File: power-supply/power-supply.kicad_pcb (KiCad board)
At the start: 2 copper layers, 25 x 11.2 mm, 12 parts, among them J1 Conn_01x04, Q1 Q_PMOS_GSD, Q3 Q_NMOS_GSD, U1 AZ1084-5.0

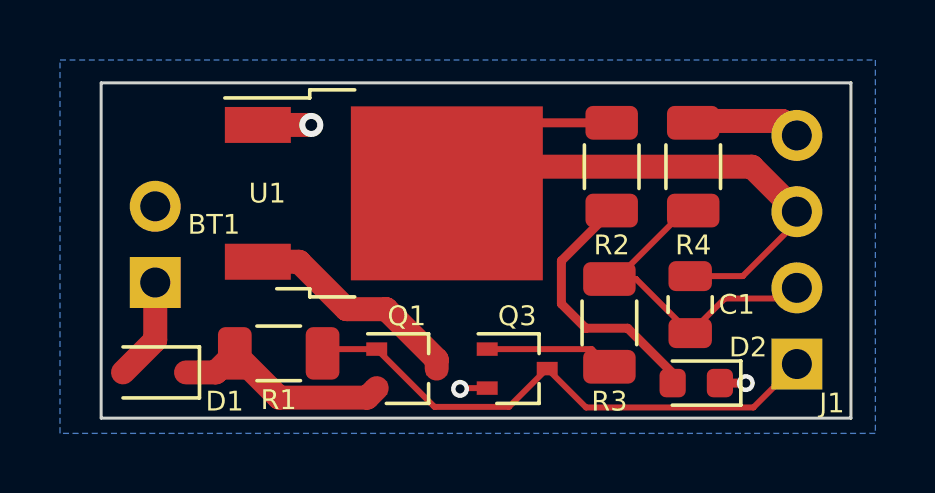
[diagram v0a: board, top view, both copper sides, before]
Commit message: misc
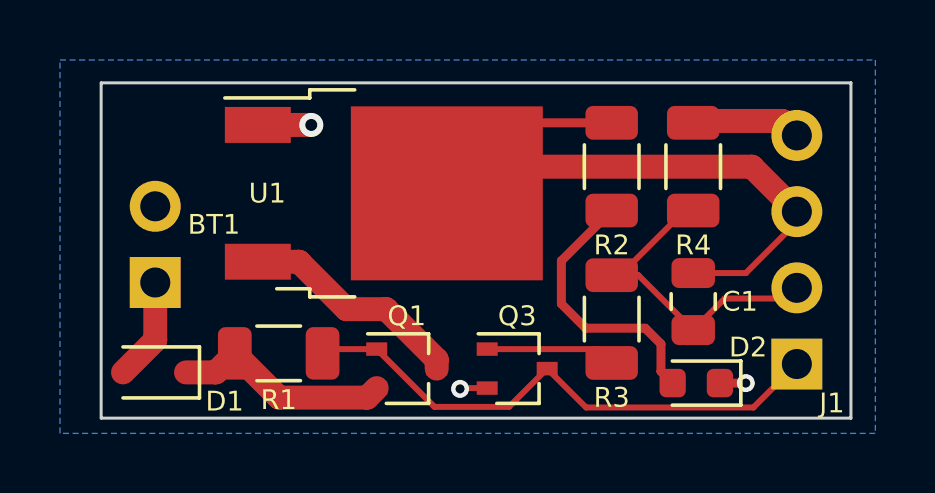
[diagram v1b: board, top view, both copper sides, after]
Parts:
- moved R3 0.15 mm to (103.7, 81.0)
- moved C1 0.14 mm to (106.5, 80.4)
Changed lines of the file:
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@@
   )
   (footprint "Resistor_SMD:R_1206_3216Metric" (layer "F.Cu")
-    (at 103.6574 81.153 90)
+    (at 103.7336 81.026 90)
     (descr "Resistor SMD 1206 (3216 Metric), square (rectangular) end terminal, IPC_7351 nominal, (Body size source: IPC-SM-782 page 72, https://www.pcb-3d.com/wordpress/wp-content/uploads/ipc-sm-782a_amendment_1_and_2.pdf), generated with kicad-footprint-generator")
     (tags "resistor")
@@
   )
   (footprint "Capacitor_SMD:C_0805_2012Metric" (layer "F.Cu")
-    (at 106.3498 80.5434 90)
+    (at 106.4514 80.4418 90)
     (descr "Capacitor SMD 0805 (2012 Metric), square (rectangular) end terminal, IPC_7351 nominal, (Body size source: IPC-SM-782 page 76, https://www.pcb-3d.com/wordpress/wp-content/uploads/ipc-sm-782a_amendment_1_and_2.pdf, https://docs.google.com/spreadsheets/d/1BsfQQcO9C6DZCsRaXUlFlo91Tg2WpOkGARC1WS5S8t0/edit?usp=sharing), generated with kicad-footprint-generator")
     (tags "capacitor")
@@
     (style (thickness 0.1) (arrow_length 1.27) (text_position_mode 0) (extension_height 0.58642) (extension_offset 0.5) keep_text_aligned)
   )
-  (segment (start 106.3498 81.4934) (end 107.503 80.3402) (width 0.2) (layer "F.Cu") (net 1))
-  (segment (start 103.6574 79.6905) (end 104.5469 79.6905) (width 0.2) (layer "F.Cu") (net 1))
-  (segment (start 103.886 79.6905) (end 103.6574 79.6905) (width 0.2) (layer "F.Cu") (net 1))
-  (segment (start 106.168 77.4085) (end 103.886 79.6905) (width 0.2) (layer "F.Cu") (net 1))
+  (segment (start 103.7336 79.5635) (end 104.6231 79.5635) (width 0.2) (layer "F.Cu") (net 1))
+  (segment (start 106.4514 77.4085) (end 106.168 77.4085) (width 0.2) (layer "F.Cu") (net 1))
   (segment (start 109.5502 80.3402) (end 109.9058 79.9846) (width 0.2) (layer "F.Cu") (net 1))
-  (segment (start 104.5469 79.6905) (end 106.3498 81.4934) (width 0.2) (layer "F.Cu") (net 1))
-  (segment (start 106.4514 77.4085) (end 106.168 77.4085) (width 0.2) (layer "F.Cu") (net 1))
+  (segment (start 104.013 79.5635) (end 103.7336 79.5635) (width 0.2) (layer "F.Cu") (net 1))
   (segment (start 107.503 80.3402) (end 109.5502 80.3402) (width 0.2) (layer "F.Cu") (net 1))
+  (segment (start 106.4514 81.3918) (end 107.503 80.3402) (width 0.2) (layer "F.Cu") (net 1))
+  (segment (start 104.6231 79.5635) (end 106.4514 81.3918) (width 0.2) (layer "F.Cu") (net 1))
+  (segment (start 106.168 77.4085) (end 104.013 79.5635) (width 0.2) (layer "F.Cu") (net 1))
+  (segment (start 108.2042 79.4918) (end 109.9058 77.7902) (width 0.2) (layer "F.Cu") (net 2))
   (segment (start 99.128 75.946) (end 108.4072 75.946) (width 0.8) (layer "F.Cu") (net 2))
   (segment (start 100.5905 74.4835) (end 98.239 76.835) (width 0.3) (layer "F.Cu") (net 2))
   (segment (start 109.9058 77.7902) (end 109.9058 77.4446) (width 0.2) (layer "F.Cu") (net 2))
   (segment (start 98.239 76.835) (end 99.128 75.946) (width 0.8) (layer "F.Cu") (net 2))
-  (segment (start 106.3498 79.5934) (end 108.1026 79.5934) (width 0.2) (layer "F.Cu") (net 2))
+  (segment (start 106.4514 79.4918) (end 108.2042 79.4918) (width 0.2) (layer "F.Cu") (net 2))
   (segment (start 108.4072 75.946) (end 109.9058 77.4446) (width 0.8) (layer "F.Cu") (net 2))
-  (segment (start 108.1026 79.5934) (end 109.9058 77.7902) (width 0.2) (layer "F.Cu") (net 2))
   (segment (start 103.7336 74.4835) (end 100.5905 74.4835) (width 0.3) (layer "F.Cu") (net 2))
   (segment (start 95.584 83.644) (end 95.901 83.327) (width 0.8) (layer "F.Cu") (net 3))
@@
   (segment (start 88.519 79.8068) (end 88.519 81.7286) (width 0.8) (layer "F.Cu") (net 7))
   (segment (start 88.519 81.7286) (end 87.4436 82.804) (width 0.8) (layer "F.Cu") (net 7))
-  (segment (start 99.584 82.027) (end 103.0689 82.027) (width 0.2) (layer "F.Cu") (net 8))
-  (segment (start 103.0689 82.027) (end 103.6574 82.6155) (width 0.2) (layer "F.Cu") (net 8))
-  (segment (start 104.267 81.3308) (end 105.7655 82.8293) (width 0.3) (layer "F.Cu") (net 9))
-  (segment (start 102.87 81.3308) (end 104.267 81.3308) (width 0.3) (layer "F.Cu") (net 9))
+  (segment (start 103.2721 82.027) (end 103.7336 82.4885) (width 0.2) (layer "F.Cu") (net 8))
+  (segment (start 99.584 82.027) (end 103.2721 82.027) (width 0.2) (layer "F.Cu") (net 8))
   (segment (start 102.0572 79.0849) (end 102.0572 80.518) (width 0.3) (layer "F.Cu") (net 9))
+  (segment (start 105.3764 81.856) (end 105.3764 82.7705) (width 0.3) (layer "F.Cu") (net 9))
+  (segment (start 105.3764 82.7705) (end 105.7655 83.1596) (width 0.3) (layer "F.Cu") (net 9))
+  (segment (start 104.8512 81.3308) (end 105.3764 81.856) (width 0.3) (layer "F.Cu") (net 9))
+  (segment (start 103.7336 77.4085) (end 102.0572 79.0849) (width 0.3) (layer "F.Cu") (net 9))
+  (segment (start 102.87 81.3308) (end 104.8512 81.3308) (width 0.3) (layer "F.Cu") (net 9))
   (segment (start 102.0572 80.518) (end 102.87 81.3308) (width 0.3) (layer "F.Cu") (net 9))
-  (segment (start 103.7336 77.4085) (end 102.0572 79.0849) (width 0.3) (layer "F.Cu") (net 9))
-  (segment (start 105.7655 82.8293) (end 105.7655 83.1596) (width 0.3) (layer "F.Cu") (net 9))
   (zone (net 6) (net_name "GND") (layer "B.Cu") (hatch edge 0.508)
     (connect_pads (clearance 0.508))
